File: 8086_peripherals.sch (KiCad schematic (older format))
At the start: 10 parts

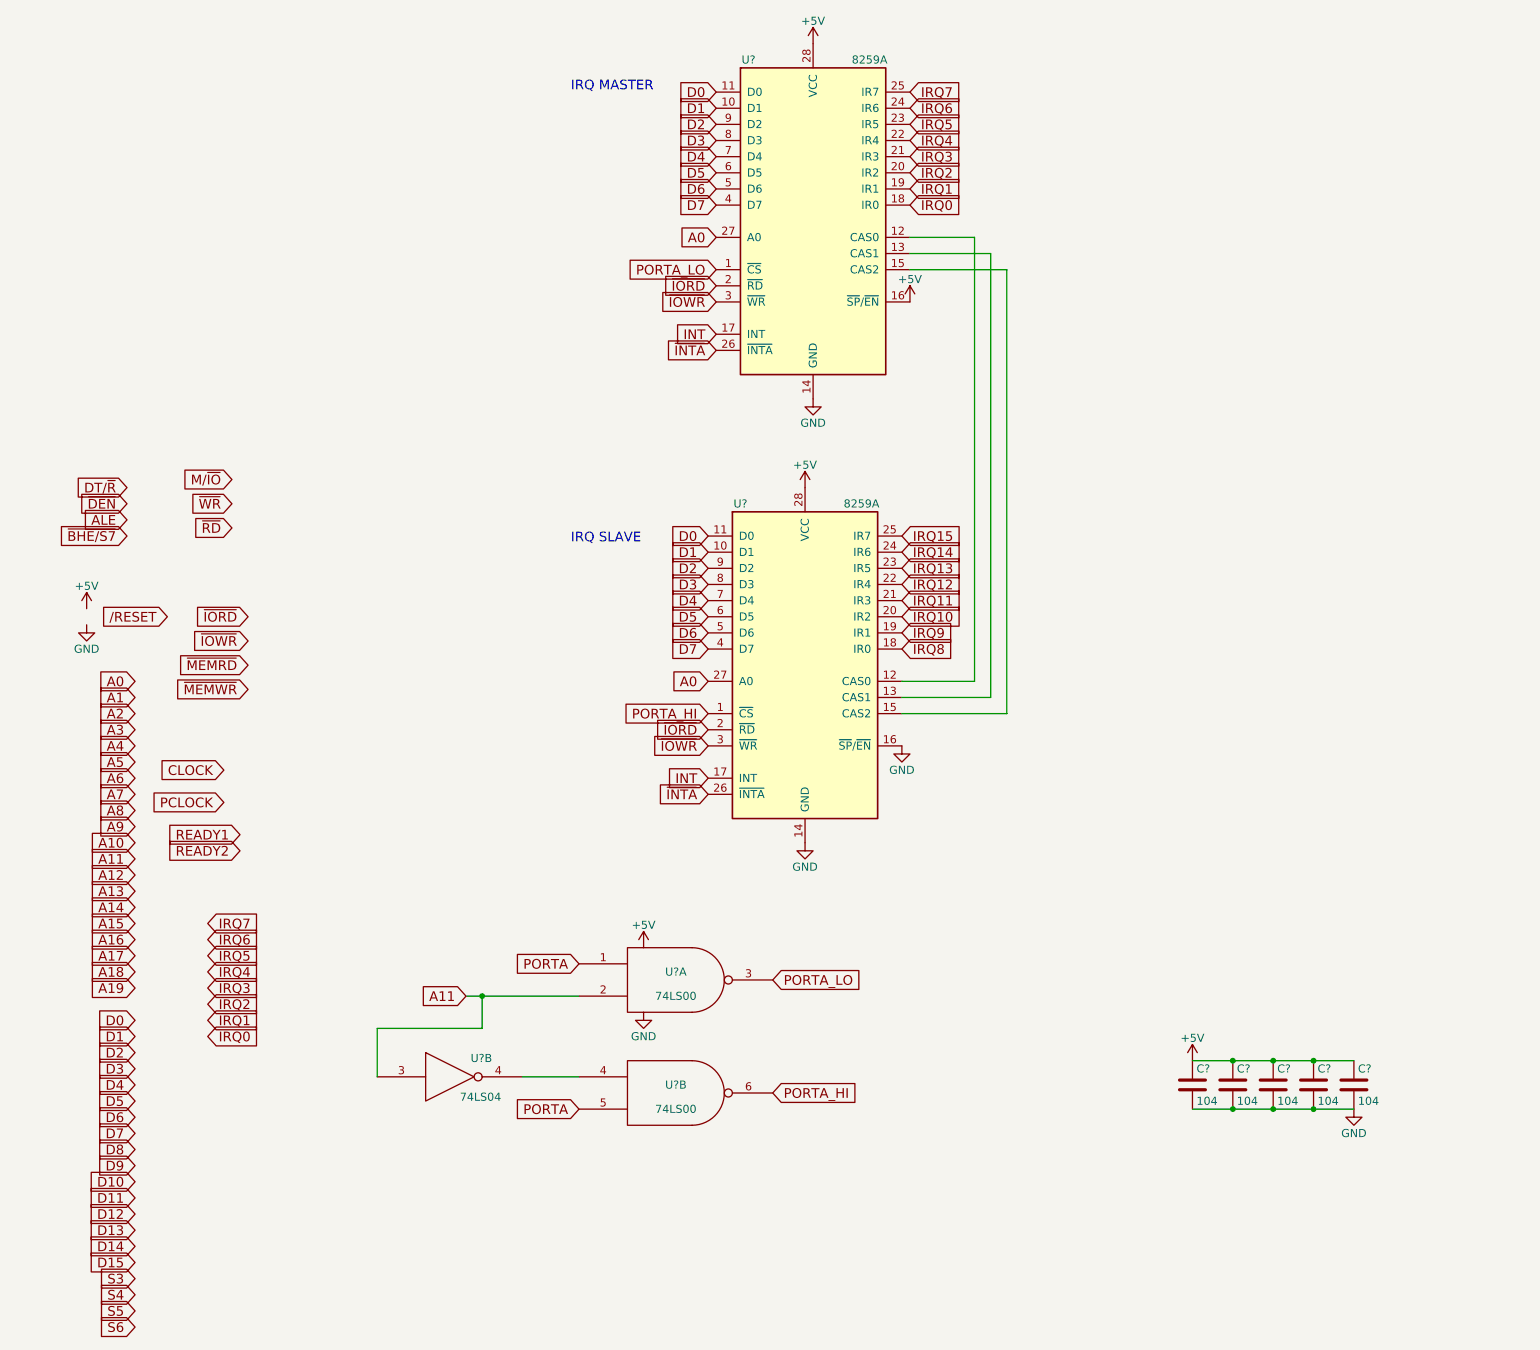
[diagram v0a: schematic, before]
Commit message: updating 8086 design
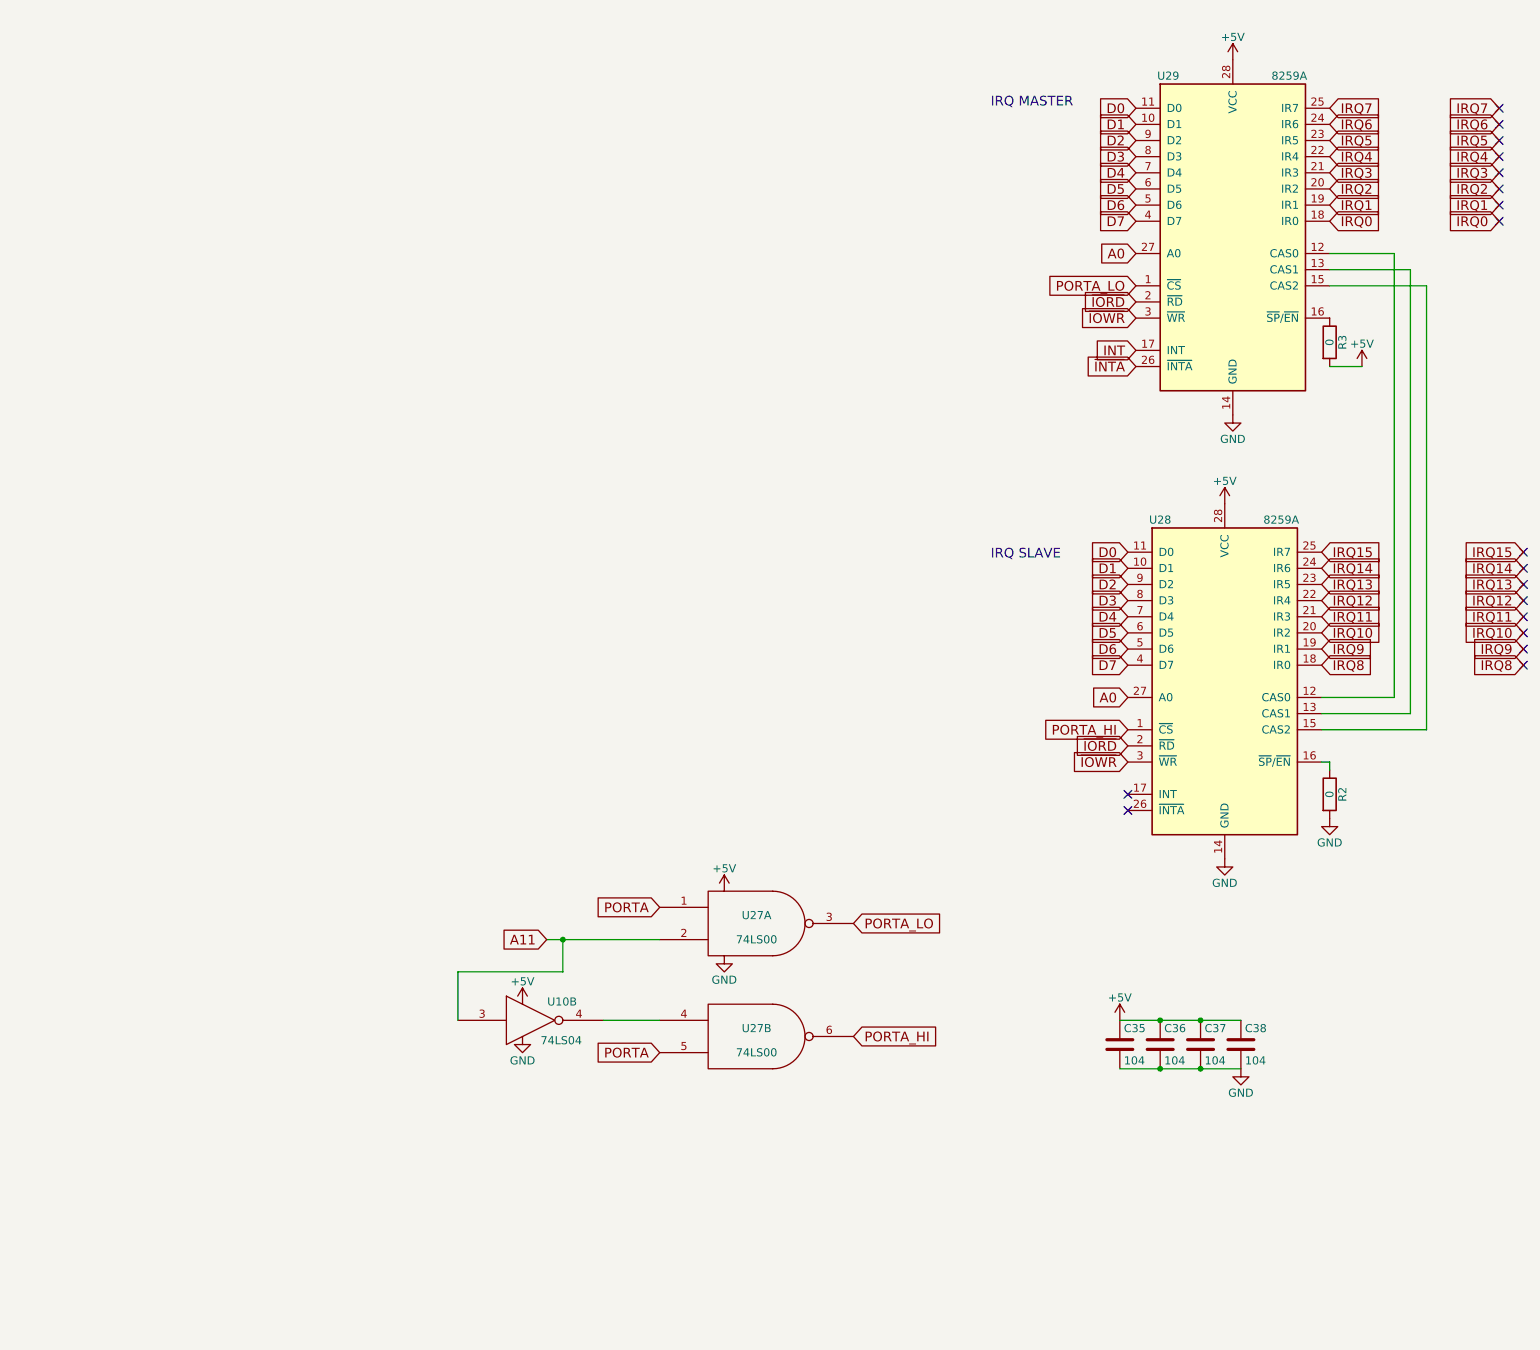
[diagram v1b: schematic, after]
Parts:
- removed C? (x5): 104, symbol C
- removed U?: 74LS04, symbol 74LS04
- added C35, C36, C37, C38: 104, symbol C
- added R2, R3: 0, symbol R
- added U10: 74LS04, symbol 74LS04
- U28, U29: renamed from U?; footprint DIP-28 -> (none)
- gave numbers to parts that had none: 1
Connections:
- net +5V: now also C35.1, C36.1, C37.1, C38.1, R3.2, U10.14 (VCC); no longer U29.16 (~SP~/~EN~)
- net A11: now also U10.3
- net GND: now also C35.2, C36.2, C37.2, C38.2, R2.2, U10.7 (GND); no longer U28.16 (~SP~/~EN~)
- net INT: no longer U28.17 (INT)
- net ~INTA: no longer U28.26 (~INTA~)
- net at U27.4: now also U10.4
- new net: R3.1, U29.16 (~SP~/~EN~)
- new net: R2.1, U28.16 (~SP~/~EN~)
- no-connect marks 0 -> 18
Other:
- moved on the sheet: U27A, U27B, U28, U29
